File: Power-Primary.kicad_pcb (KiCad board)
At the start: 2 copper layers, 174 x 72 mm, 53 parts, among them J1 HV in, J10 SPARE, J11 SPARE, J2 Dashboard, J3 Telemetry, J4 Motor, J5 MPPT 1, J6 MPPT 2, J7 BPS, J8 Primary Disconn., J9 SPARE, U1 Mean_Well_12V

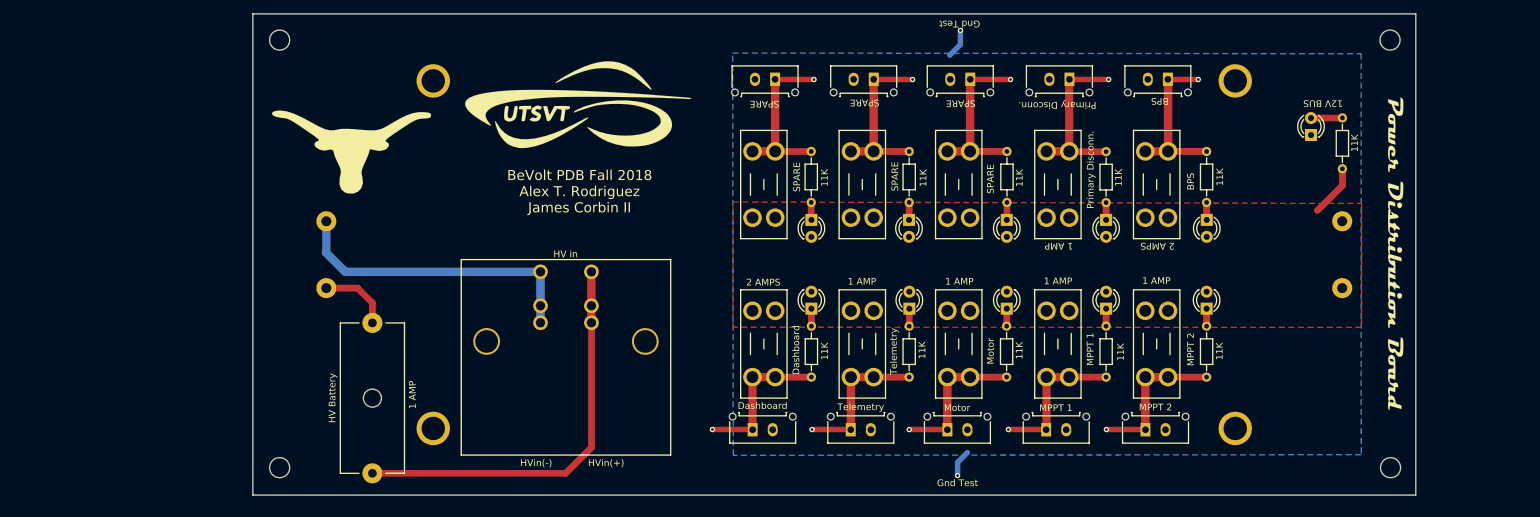
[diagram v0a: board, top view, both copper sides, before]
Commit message: finished PCB waiting for edits
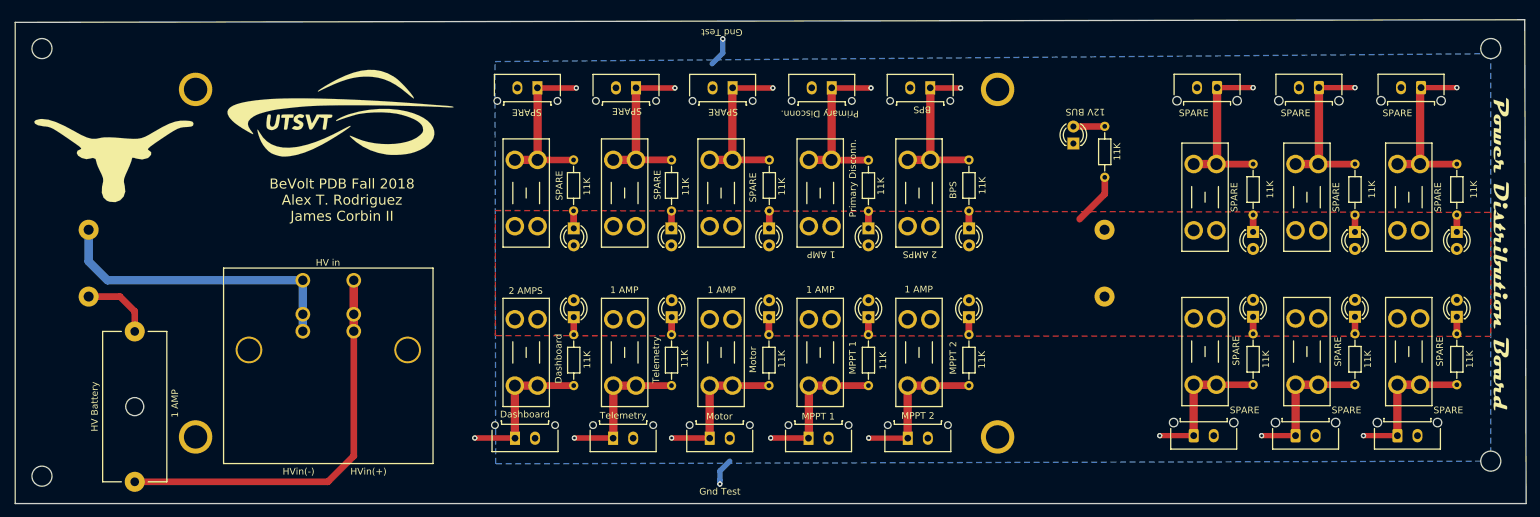
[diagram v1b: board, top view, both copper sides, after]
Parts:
- added D11: LED, LED_THT:LED_D3.0mm, F.Cu at (200.7, 100.3)
- added D12: LED, LED_THT:LED_D3.0mm, F.Cu at (215.9, 100.3)
- added D13: LED, LED_THT:LED_D3.0mm, F.Cu at (231.1, 100.3)
- added D14: LED, LED_THT:LED_D3.0mm, F.Cu at (231.1, 87.6)
- added D15: LED, LED_THT:LED_D3.0mm, F.Cu at (215.9, 87.6)
- added D16: LED, LED_THT:LED_D3.0mm, F.Cu at (200.7, 87.6)
- added F12: SPARE, Fuse:Fuseholder_Blade_Mini_Keystone_3568, F.Cu at (195.2, 100.6)
- added F13: SPARE, Fuse:Fuseholder_Blade_Mini_Keystone_3568, F.Cu at (210.4, 100.6)
- added F14: SPARE, Fuse:Fuseholder_Blade_Mini_Keystone_3568, F.Cu at (225.7, 100.6)
- added F15: SPARE, Fuse:Fuseholder_Blade_Mini_Keystone_3568, F.Cu at (222.2, 87.4)
- added F16: SPARE, Fuse:Fuseholder_Blade_Mini_Keystone_3568, F.Cu at (207.0, 87.4)
- added F17: SPARE, Fuse:Fuseholder_Blade_Mini_Keystone_3568, F.Cu at (191.8, 87.4)
- added J12: SPARE, Connector_Molex:Molex_Micro-Fit_3.0_43650-0215_1x02_P3.00mm_Vertical, F.Cu at (191.8, 118.1)
- added J13: SPARE, Connector_Molex:Molex_Micro-Fit_3.0_43650-0215_1x02_P3.00mm_Vertical, F.Cu at (207.0, 118.1)
- added J14: SPARE, Connector_Molex:Molex_Micro-Fit_3.0_43650-0215_1x02_P3.00mm_Vertical, F.Cu at (222.2, 118.1)
- added J15: SPARE, Connector_Molex:Molex_Micro-Fit_3.0_43650-0215_1x02_P3.00mm_Vertical, F.Cu at (225.8, 66.0)
- added J16: SPARE, Connector_Molex:Molex_Micro-Fit_3.0_43650-0215_1x02_P3.00mm_Vertical, F.Cu at (210.5, 66.0)
- added J17: SPARE, Connector_Molex:Molex_Micro-Fit_3.0_43650-0215_1x02_P3.00mm_Vertical, F.Cu at (195.3, 66.0)
- added R11: 11K, Resistor_THT:R_Axial_DIN0204_L3.6mm_D1.6mm_P7.62mm_Horizontal, F.Cu at (200.7, 110.5)
- added R12: 11K, Resistor_THT:R_Axial_DIN0204_L3.6mm_D1.6mm_P7.62mm_Horizontal, F.Cu at (215.9, 110.5)
- added R13: 11K, Resistor_THT:R_Axial_DIN0204_L3.6mm_D1.6mm_P7.62mm_Horizontal, F.Cu at (231.1, 110.5)
- added R14: 11K, Resistor_THT:R_Axial_DIN0204_L3.6mm_D1.6mm_P7.62mm_Horizontal, F.Cu at (231.1, 77.5)
- added R15: 11K, Resistor_THT:R_Axial_DIN0204_L3.6mm_D1.6mm_P7.62mm_Horizontal, F.Cu at (215.9, 77.5)
- added R16: 11K, Resistor_THT:R_Axial_DIN0204_L3.6mm_D1.6mm_P7.62mm_Horizontal, F.Cu at (200.7, 77.5)
- moved D9 35.6 mm to (113.6, 89.6)
- moved F3 35.6 mm to (108.3, 100.7)
- moved F4 35.6 mm to (122.8, 100.7)
- moved J1 35.6 mm to (58.5, 94.9)
- moved D17 35.6 mm to (173.8, 74.4)
- moved D3 35.6 mm to (128.2, 97.8)
- moved D4 35.6 mm to (143.1, 97.8)
- moved D5 35.6 mm to (158.1, 97.8)
- moved D6 35.6 mm to (158.2, 89.6)
- moved D7 35.6 mm to (143.1, 89.6)
- moved D8 35.6 mm to (128.2, 89.6)
- moved F10 35.6 mm to (104.9, 86.8)
- moved F5 35.6 mm to (137.6, 100.7)
- moved F6 35.6 mm to (152.4, 100.7)
- moved F7 35.6 mm to (149.0, 86.8)
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- renumbered D11 to D17, R11 to R18
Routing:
- net Net-(F16-Pad2): track 0.00 -> 25.8 mm, vias 0 -> 1
- net Net-(F17-Pad2): track 0.00 -> 25.8 mm, vias 0 -> 1
- net Net-(F15-Pad2): track 0.00 -> 25.7 mm, vias 0 -> 1
- net Net-(F14-Pad2): track 0.00 -> 21.6 mm, vias 0 -> 1
- net Net-(F13-Pad2): track 0.00 -> 21.6 mm, vias 0 -> 1
- net Net-(F12-Pad2): track 0.00 -> 21.6 mm, vias 0 -> 1
- net Net-(D13-Pad2): track 0.00 -> 2.54 mm
- net Net-(D12-Pad2): track 0.00 -> 2.54 mm
- net Net-(D11-Pad2): track 0.00 -> 2.54 mm
- net Net-(D16-Pad2): track 0.00 -> 2.54 mm
- net Net-(D15-Pad2): track 0.00 -> 2.54 mm
- net Net-(D14-Pad2): track 0.00 -> 2.54 mm
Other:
- board size 174 x 72 mm -> 226.1 x 72.4 mm

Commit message: pcb edits
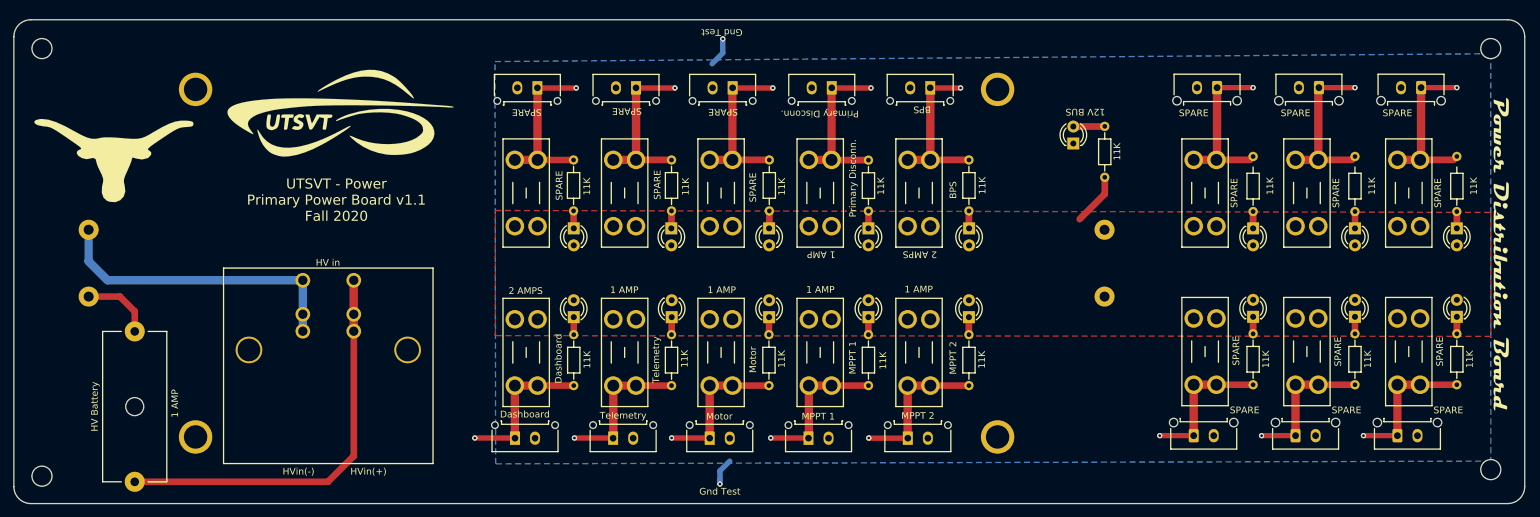
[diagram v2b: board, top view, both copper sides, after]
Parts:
- moved REF** 1.27 mm to (236.2, 123.2)
- moved F15 0.62 mm to (222.2, 86.8)
- moved F16 0.62 mm to (207.0, 86.8)
- moved F17 0.62 mm to (191.8, 86.8)
- moved D14 0.53 mm to (231.1, 87.1)
- moved D15 0.53 mm to (215.9, 87.1)
- moved D16 0.53 mm to (200.7, 87.1)
- moved R14 0.51 mm to (231.1, 77.0)
- moved R15 0.51 mm to (215.9, 77.0)
- moved R16 0.51 mm to (200.7, 77.0)
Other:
- outline, holes or cut-outs redrawn
- board text added: "UTSVT - Power Primary Power Board v1.1 Fall 2020"
- board text removed: "BeVolt PDB Fall 2018 Alex T. Rodriguez James Corbin II"
